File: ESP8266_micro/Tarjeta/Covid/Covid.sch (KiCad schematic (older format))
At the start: 12 parts, among them U1 ESP32, U10 SOURCE, U2 LASER, U3 AMPLIFICADOR, U4 Trinket_M0, U5 JQ6500-16P, U6 L7805, U7 Boton_IR, U8 Boton_IR, U9 MLX90614

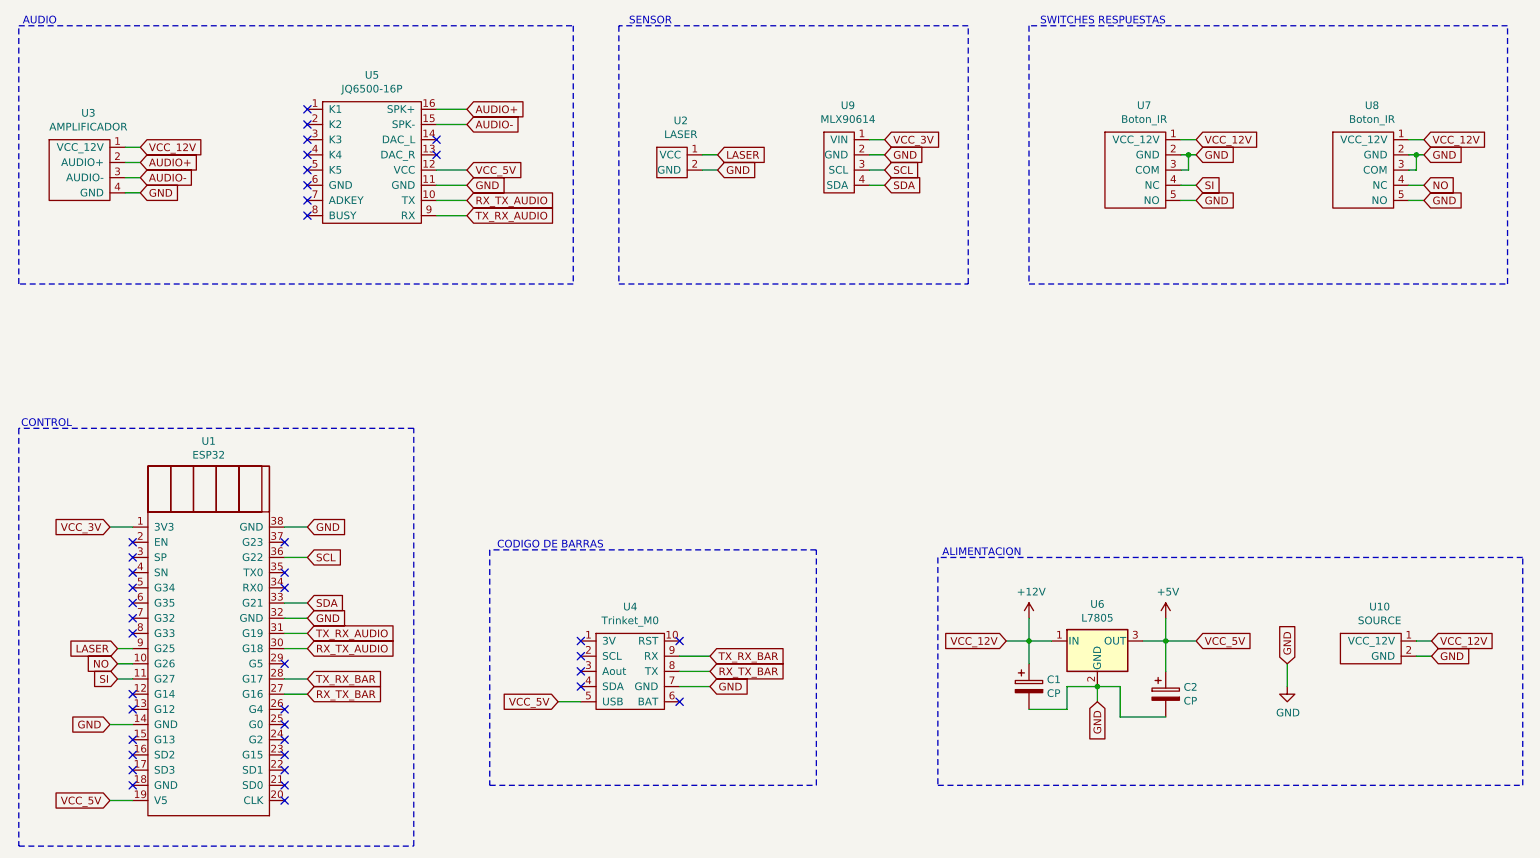
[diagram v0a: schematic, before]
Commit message: PCB con Pantalla SPI
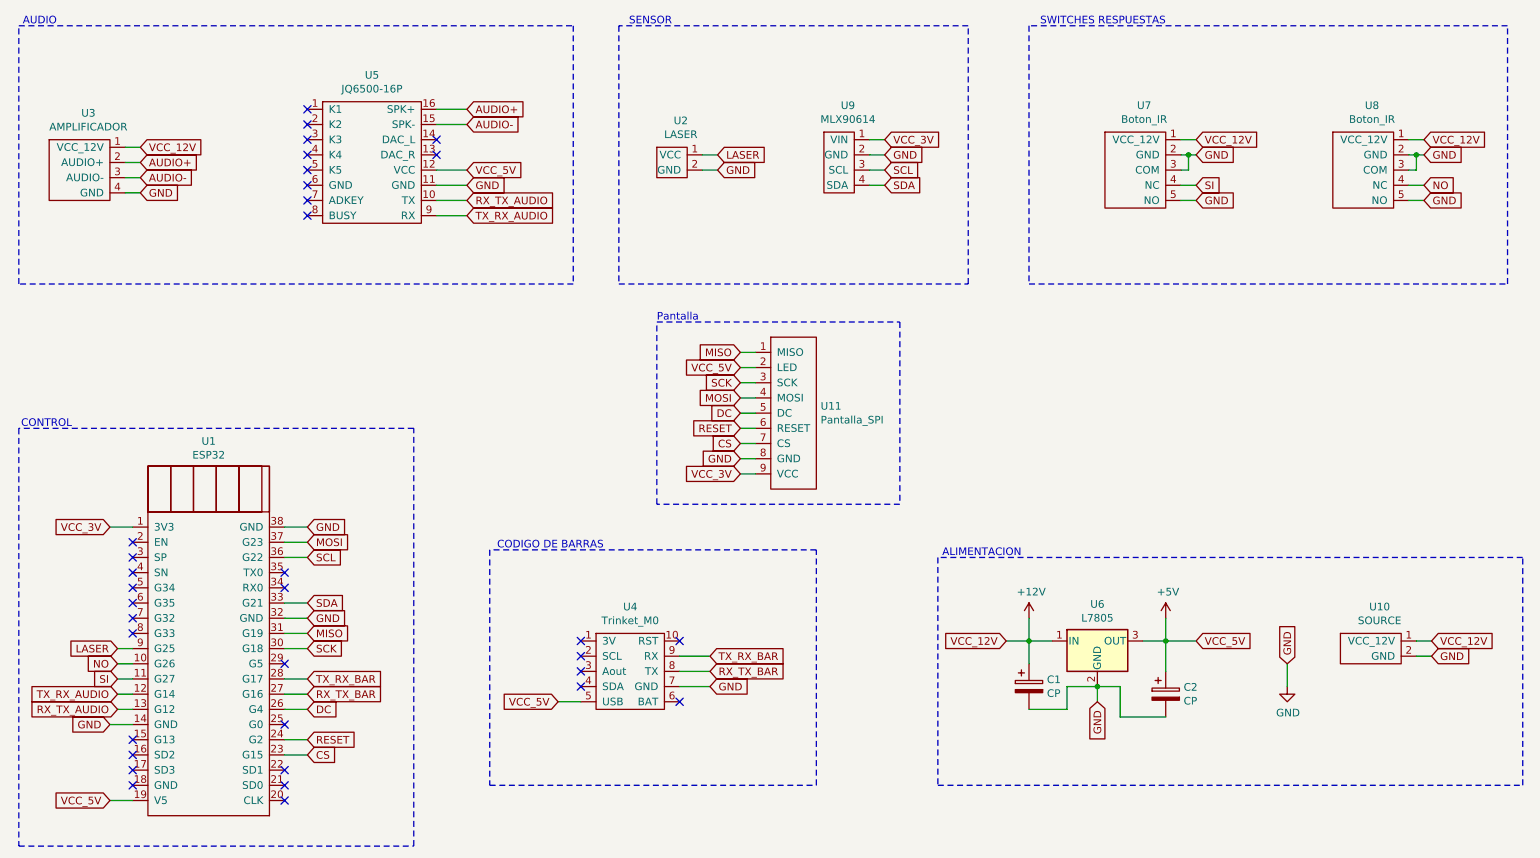
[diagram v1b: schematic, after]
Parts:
- added U11: Pantalla_SPI, Covid:Pantalla_spi, symbol covid:Pantalla_SPI
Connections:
- net +5V: now also U11.2 (LED)
- net GND: now also U11.8 (GND)
- net RX_TX_AUDIO: now also U1.13 (G12); no longer U1.30 (G18)
- net TX_RX_AUDIO: now also U1.12 (G14); no longer U1.31 (G19)
- net VCC_3V: now also U11.9 (VCC)
- net CS: now reaches U1.23 (G15)
- net CS: now also U11.7 (CS)
- net RESET: now reaches U1.24 (G2)
- net RESET: now also U11.6 (RESET)
- net DC: now reaches U1.26 (G4)
- net DC: now also U11.5 (DC)
- net MOSI: now reaches U1.37 (G23)
- net MOSI: now also U11.4 (MOSI)
- new net MISO: U1.31 (G19), U11.1 (MISO)
- new net SCK: U1.30 (G18), U11.3 (SCK)
- no-connect marks 40 -> 34
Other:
- note added: "Pantalla"
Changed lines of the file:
@@
 Wire Wire Line
 	9200 5200 9200 5350
-Text GLabel 2750 5000 2    50   Input ~ 0
+Text GLabel 1500 5400 0    50   Input ~ 0
 TX_RX_AUDIO
 Text GLabel 3800 2250 2    50   Input ~ 0
@@
 Wire Wire Line
 	2750 5000 2600 5000
-Text GLabel 2750 5100 2    50   Input ~ 0
+Text GLabel 1500 5500 0    50   Input ~ 0
 RX_TX_AUDIO
 Text GLabel 3800 2150 2    50   Input ~ 0
@@
 NoConn ~ 4550 5150
 NoConn ~ 4550 5050
-NoConn ~ 2600 4400
 NoConn ~ 2600 4600
 NoConn ~ 2600 4700
 NoConn ~ 2600 5200
-NoConn ~ 2600 5500
 NoConn ~ 2600 5600
-NoConn ~ 2600 5700
-NoConn ~ 2600 5800
 NoConn ~ 2600 5900
 NoConn ~ 2600 6000
@@
 NoConn ~ 1600 5700
 NoConn ~ 1600 5800
-NoConn ~ 1600 5500
-NoConn ~ 1600 5400
 NoConn ~ 1600 5000
 NoConn ~ 1600 4900
@@
 SWITCHES RESPUESTAS\n
 NoConn ~ 2750 2050
+Wire Wire Line
+	1500 5400 1600 5400
+Wire Wire Line
+	1500 5500 1600 5500
+Text GLabel 2750 4400 2    50   Input ~ 0
+MOSI
+Wire Wire Line
+	2600 4400 2750 4400
+Text GLabel 2750 5000 2    50   Input ~ 0
+MISO
+Text GLabel 2750 5100 2    50   Input ~ 0
+SCK
+$Comp
+L covid:Pantalla_SPI U11
+U 1 1 5F03D09D
+P 5550 3050
+F 0 "U11" H 6128 2596 50  0000 L CNN
+F 1 "Pantalla_SPI" H 6128 2505 50  0000 L CNN
+F 2 "Covid:Pantalla_spi" H 5550 3050 50  0001 C CNN
+F 3 "" H 5550 3050 50  0001 C CNN
+	1    5550 3050
+	1    0    0    -1
+$EndComp
+Text GLabel 5600 3150 0    50   Input ~ 0
+MISO
+Text GLabel 5600 3250 0    50   Input ~ 0
+VCC_5V
+Text GLabel 5600 3350 0    50   Input ~ 0
+SCK
+Text GLabel 5600 3450 0    50   Input ~ 0
+MOSI
+Text GLabel 5600 3550 0    50   Input ~ 0
+DC
+Text GLabel 5600 3650 0    50   Input ~ 0
+RESET
+Text GLabel 5600 3750 0    50   Input ~ 0
+CS
+Text GLabel 5600 3850 0    50   Input ~ 0
+GND
+Text GLabel 5600 3950 0    50   Input ~ 0
+VCC_3V
+Wire Wire Line
+	5600 3150 5700 3150
+Wire Wire Line
+	5600 3250 5700 3250
+Wire Wire Line
+	5600 3350 5700 3350
+Wire Wire Line
+	5600 3450 5700 3450
+Wire Wire Line
+	5600 3550 5700 3550
+Wire Wire Line
+	5600 3650 5700 3650
+Wire Wire Line
+	5600 3750 5700 3750
+Wire Wire Line
+	5600 3850 5700 3850
+Wire Wire Line
+	5600 3950 5700 3950
+Wire Notes Line
+	5050 2950 6650 2950
+Wire Notes Line
+	6650 2950 6650 4150
+Wire Notes Line
+	6650 4150 5050 4150
+Wire Notes Line
+	5050 4150 5050 2950
+Text Notes 5050 2950 0    50   ~ 0
+Pantalla
+Text GLabel 2750 5800 2    50   Input ~ 0
+CS
+Text GLabel 2750 5700 2    50   Input ~ 0
+RESET
+Text GLabel 2750 5500 2    50   Input ~ 0
+DC
+Wire Wire Line
+	2600 5500 2750 5500
+Wire Wire Line
+	2600 5700 2750 5700
+Wire Wire Line
+	2600 5800 2750 5800
 $EndSCHEMATC

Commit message: pcb
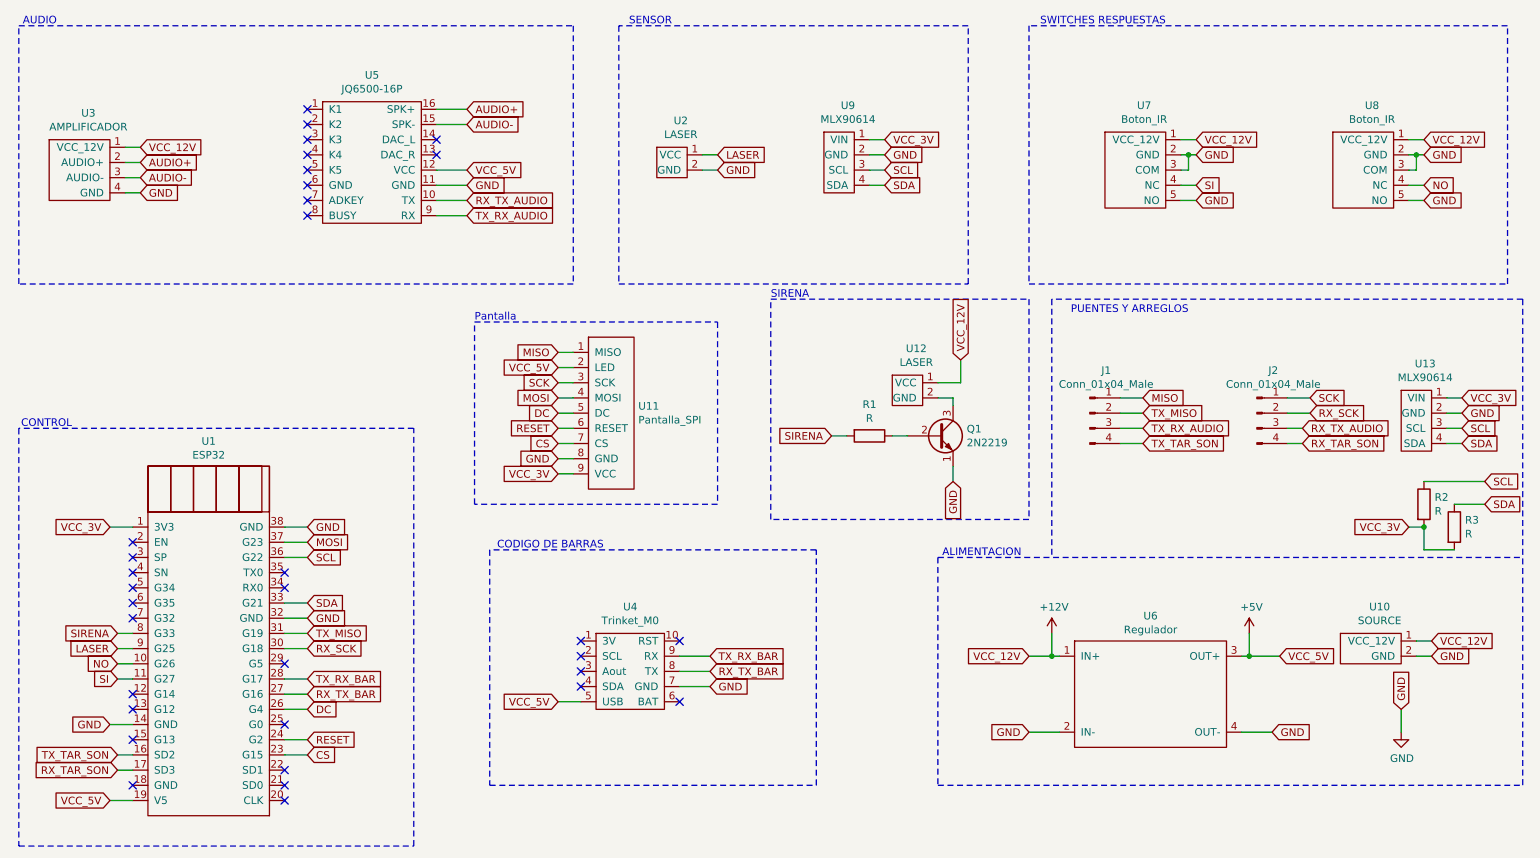
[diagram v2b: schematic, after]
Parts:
- removed C1, C2: CP, Covid:CAP_1uf, symbol Device:CP
- removed U6: L7805, Converter_DCDC:Converter_DCDC_muRata_OKI-78SR_Vertical, symbol Regulator_Linear:L7805
- added J1, J2: Conn_01x04_Male, TerminalBlock_TE-Connectivity:TerminalBlock_TE_282834-4_1x04_P2.54mm_Horizontal, symbol Connector:Conn_01x04_Male
- added Q1: 2N2219, Package_TO_SOT_THT:TO-92L_Inline, symbol Transistor_BJT:2N2219
- added R1, R2, R3: R, Resistor_THT:R_Axial_DIN0309_L9.0mm_D3.2mm_P2.54mm_Vertical, symbol Device:R
- added U12: LASER, Covid:LASER, symbol covid:LASER
- added U13: MLX90614, TerminalBlock_TE-Connectivity:TerminalBlock_TE_282834-4_1x04_P2.54mm_Horizontal, symbol covid:MLX90614
- added U6: Regulador, Covid:Regulador, symbol covid:Regulador
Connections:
- net +12V: now also U12.1 (VCC), U6.1 (IN+)
- net +5V: now also U6.3 (OUT+)
- net GND: now also Q1.1 (E), U13.2 (GND), U6.2 (IN-), U6.4 (OUT-)
- net MISO: now also J1.1 (Pin_1); no longer U1.31 (G19)
- net RX_TX_AUDIO: now also J2.3 (Pin_3); no longer U1.13 (G12)
- net SCK: now also J2.1 (Pin_1); no longer U1.30 (G18)
- net SCL: now also R2.1, U13.3 (SCL)
- net SDA: now also R3.1, U13.4 (SDA)
- net TX_RX_AUDIO: now also J1.3 (Pin_3); no longer U1.12 (G14)
- net VCC_3V: now also R2.2, R3.2, U13.1 (VIN)
- net TX_TAR_SON: now reaches U1.16 (SD2)
- net TX_TAR_SON: now also J1.4 (Pin_4)
- net RX_TAR_SON: now reaches U1.17 (SD3)
- net RX_TAR_SON: now also J2.4 (Pin_4)
- net SIRENA: now reaches U1.8 (G33)
- net SIRENA: now also R1.2
- new net: Q1.2 (B), R1.1
- new net: Q1.3 (C), U12.2 (GND)
- new net RX_SCK: J2.2 (Pin_2), U1.30 (G18)
- new net TX_MISO: J1.2 (Pin_2), U1.31 (G19)
- no-connect marks 34 -> 33
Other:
- note added: "PUENTES Y ARREGLOS\n"
- note added: "SIRENA\n"
- moved on the sheet: U11
